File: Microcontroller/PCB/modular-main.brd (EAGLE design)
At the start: 62.2 x 44.1 mm, 16 parts, among them IC1 7805T

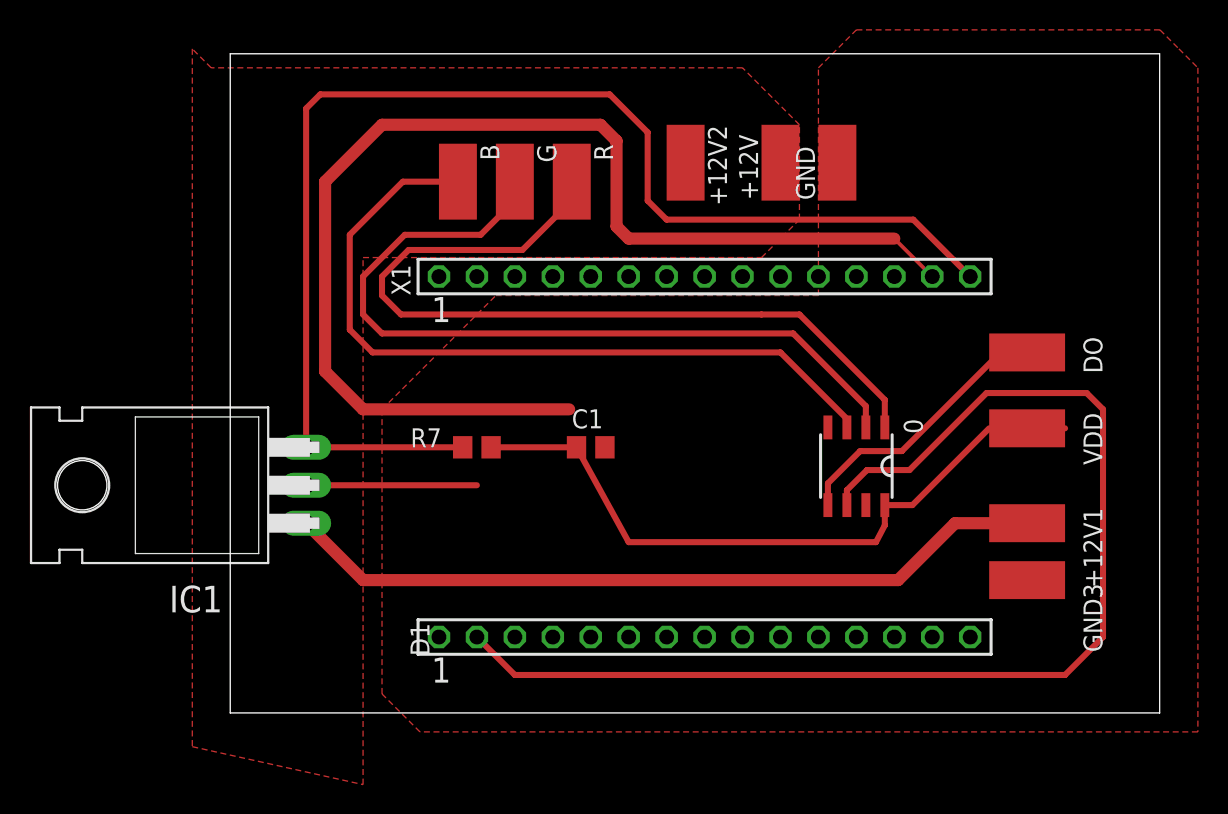
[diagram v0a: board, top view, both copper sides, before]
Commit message: Added MARKII PCB designs
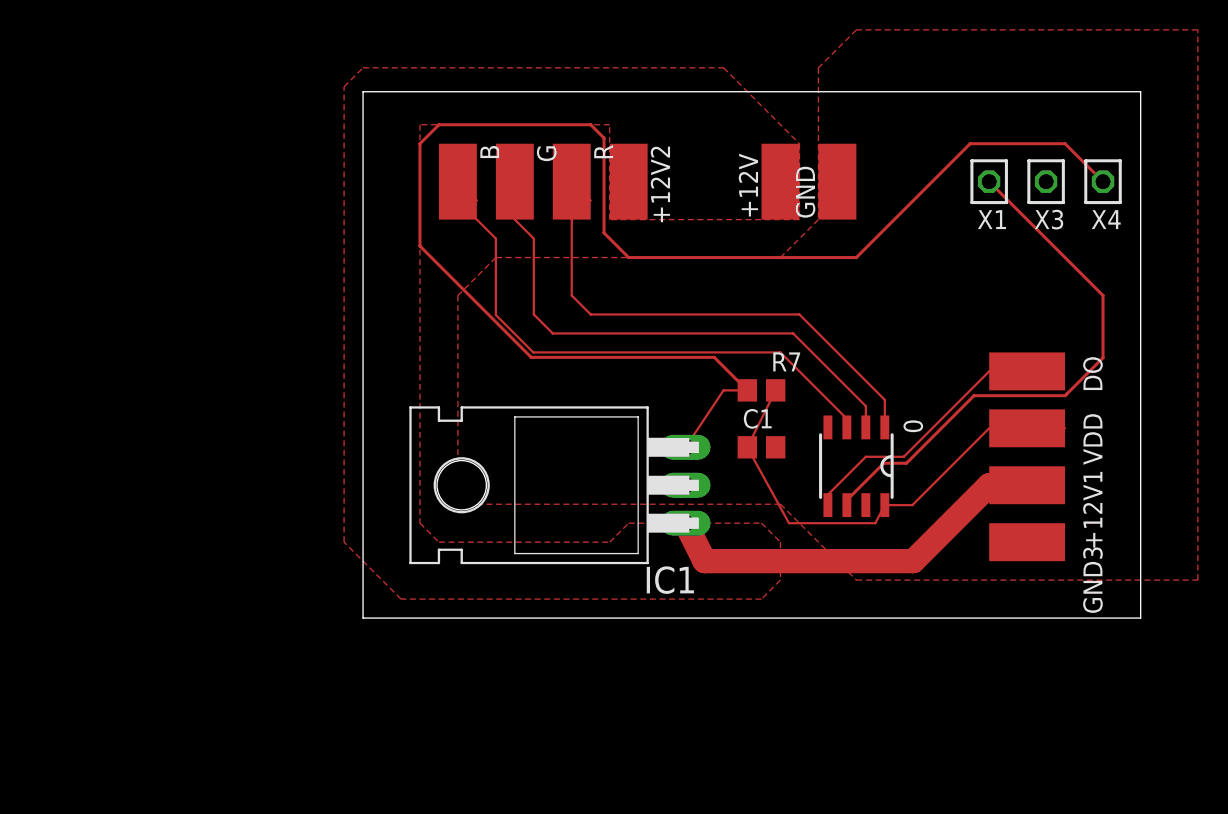
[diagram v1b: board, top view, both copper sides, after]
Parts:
- removed D1: (no value), con-samtec:SSW-115-02-G-S
- added X3: GND, con-samtec:SSW-101-02-G-S
- added X4: VDD, con-samtec:SSW-101-02-G-S
- X1: value (none) -> D1; device con-samtec:SSW-115-02-G-S -> con-samtec:SSW-101-02-G-S
- moved IC1 25.4 mm to (12.7, 20.3)
- moved X1 20.1 mm to (43.2, 40.6), turned to 90 degrees
- moved R7 19.4 mm to (27.9, 26.7)
- moved C1 11.4 mm to (27.9, 22.9)
- moved +12V2 4.02 mm to (19.1, 40.6)
- moved GND3 2.54 mm to (45.7, 16.5)
- moved +12V1 2.54 mm to (45.7, 20.3)
- moved DO 1.27 mm to (45.7, 27.9)
- moved +12V 1.27 mm to (29.2, 40.6)
- moved GND 1.27 mm to (33.0, 40.6)
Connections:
- net GND: now also X3.1; no longer X1.14
- net N$1: now also X1.1; no longer D1.2
- net N$28: now also X4.1; no longer X1.15
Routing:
- net GND: track 91.3 -> 0.00 mm
- net N$1: track 80.5 -> 36.4 mm
- net N$29: track 51.4 -> 26.5 mm
- net N$5: track 55.7 -> 35.1 mm
- net N$4: track 53.2 -> 35.6 mm
- net +5V: track 43.8 -> 28.9 mm
- net N$3: track 51.4 -> 37.5 mm
- net N$28: track 85.7 -> 96.8 mm
- net N$2: track 18.5 -> 17.5 mm
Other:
- board size 62.2 x 44.1 mm -> 52 x 35.2 mm
